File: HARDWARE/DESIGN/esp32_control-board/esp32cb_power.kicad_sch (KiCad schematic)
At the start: 31 parts, among them J101 Power-in, Q101 AO4407C, Q102 DMP3013SFV-7, U101 LM63615DQDRRRQ1, U102 AMS1117-3.3

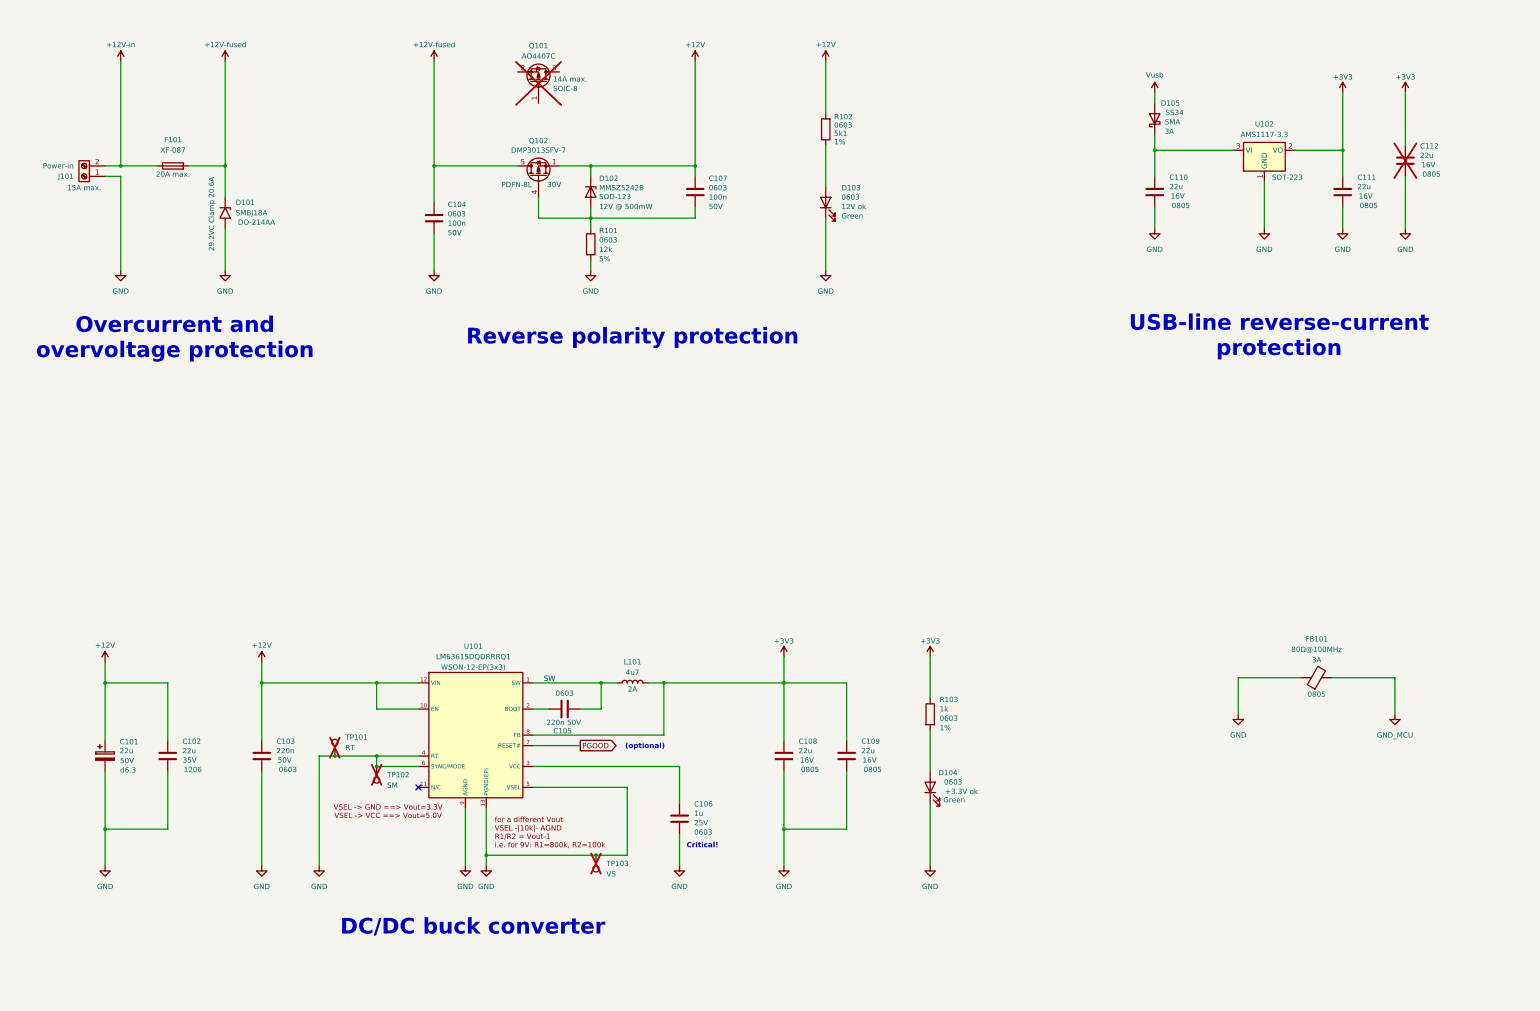
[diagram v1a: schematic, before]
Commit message: 60825 - Schematic update and PCB-layout started
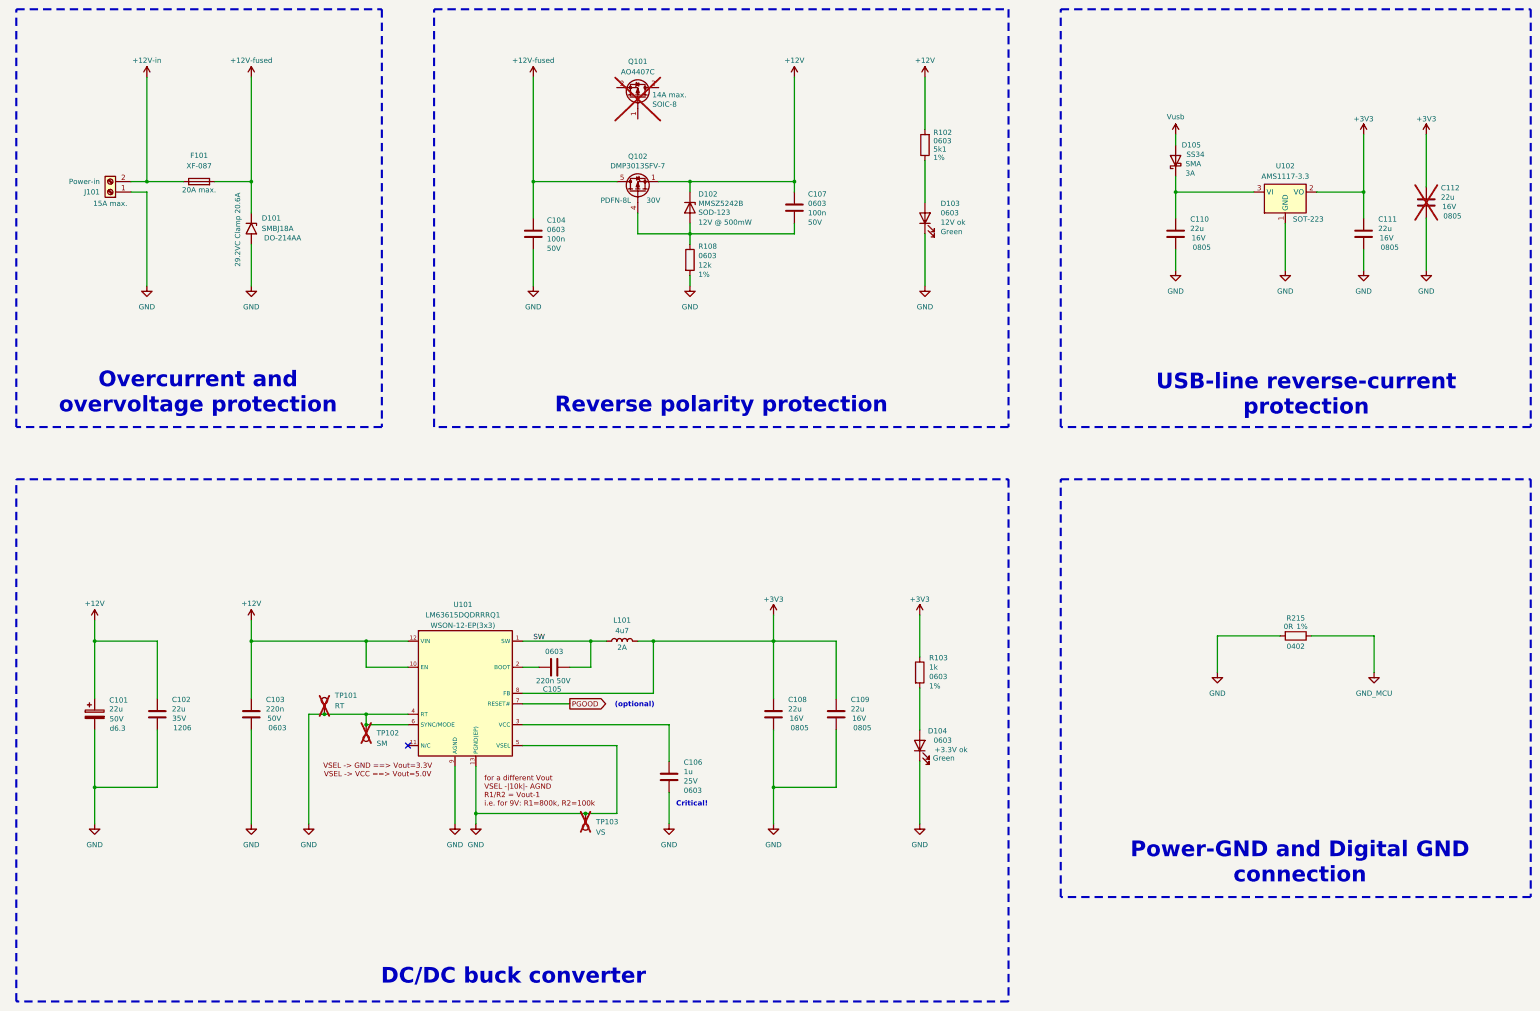
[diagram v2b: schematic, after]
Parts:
- removed FB101: 80Ω@100MHz, Inductor_SMD:L_0805_2012Metric, symbol Device:FerriteBead
- removed R101: 12k, Resistor_SMD:R_0603_1608Metric, symbol Device:R
- added R108: 12k, Resistor_SMD:R_0603_1608Metric, symbol Device:R
- added R215: 0R, Resistor_SMD:R_0402_1005Metric, symbol Device:R
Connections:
- net GND: now also R108.2, R215.2
- net GND_MCU: now also R215.1
- net at C107.1, D102.2 (A), Q102.4 (G): now also R108.1
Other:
- note added: "Power-GND and Digital GND connection"
- moved on the sheet: C101, C102, C103, C104, C105, C106, C107, C108, C109, C110, C111, C112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
